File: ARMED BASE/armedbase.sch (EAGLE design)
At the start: 20 parts, among them IC1 REG1117, K1 CQ1-12V, X1 RJ45-6L2-B, X2 RJ45-6L2-B, X3 14867

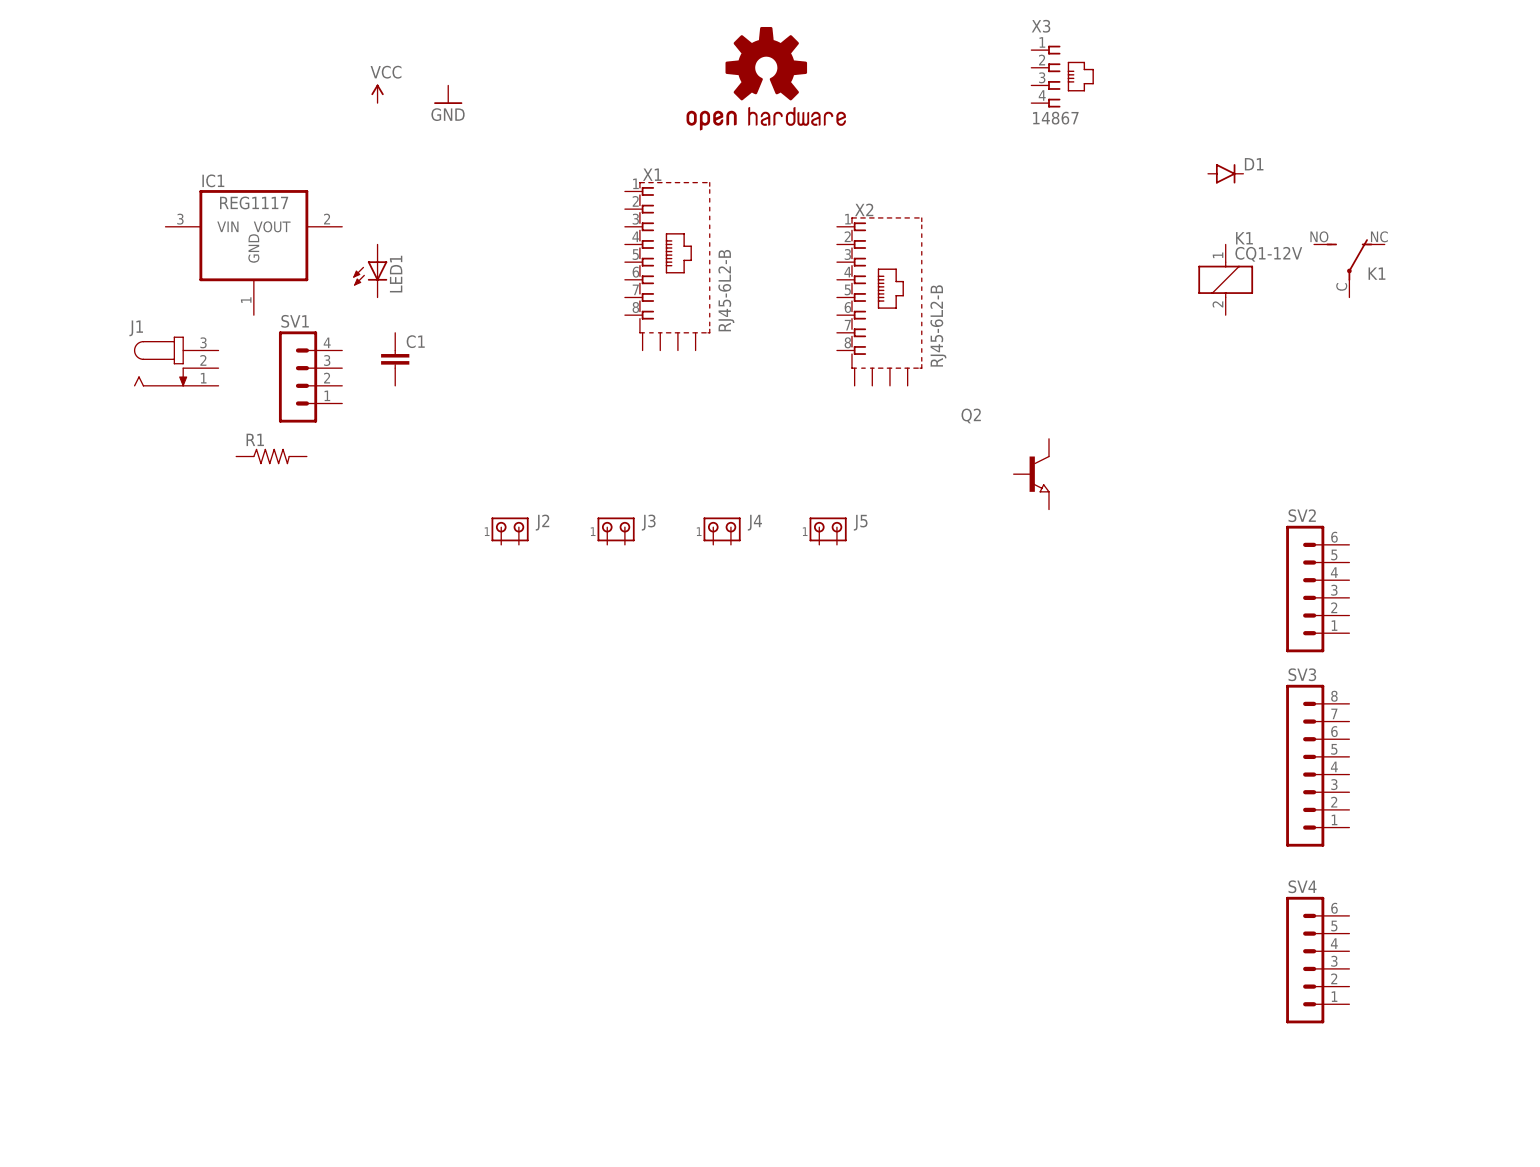
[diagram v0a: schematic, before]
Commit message: modbus
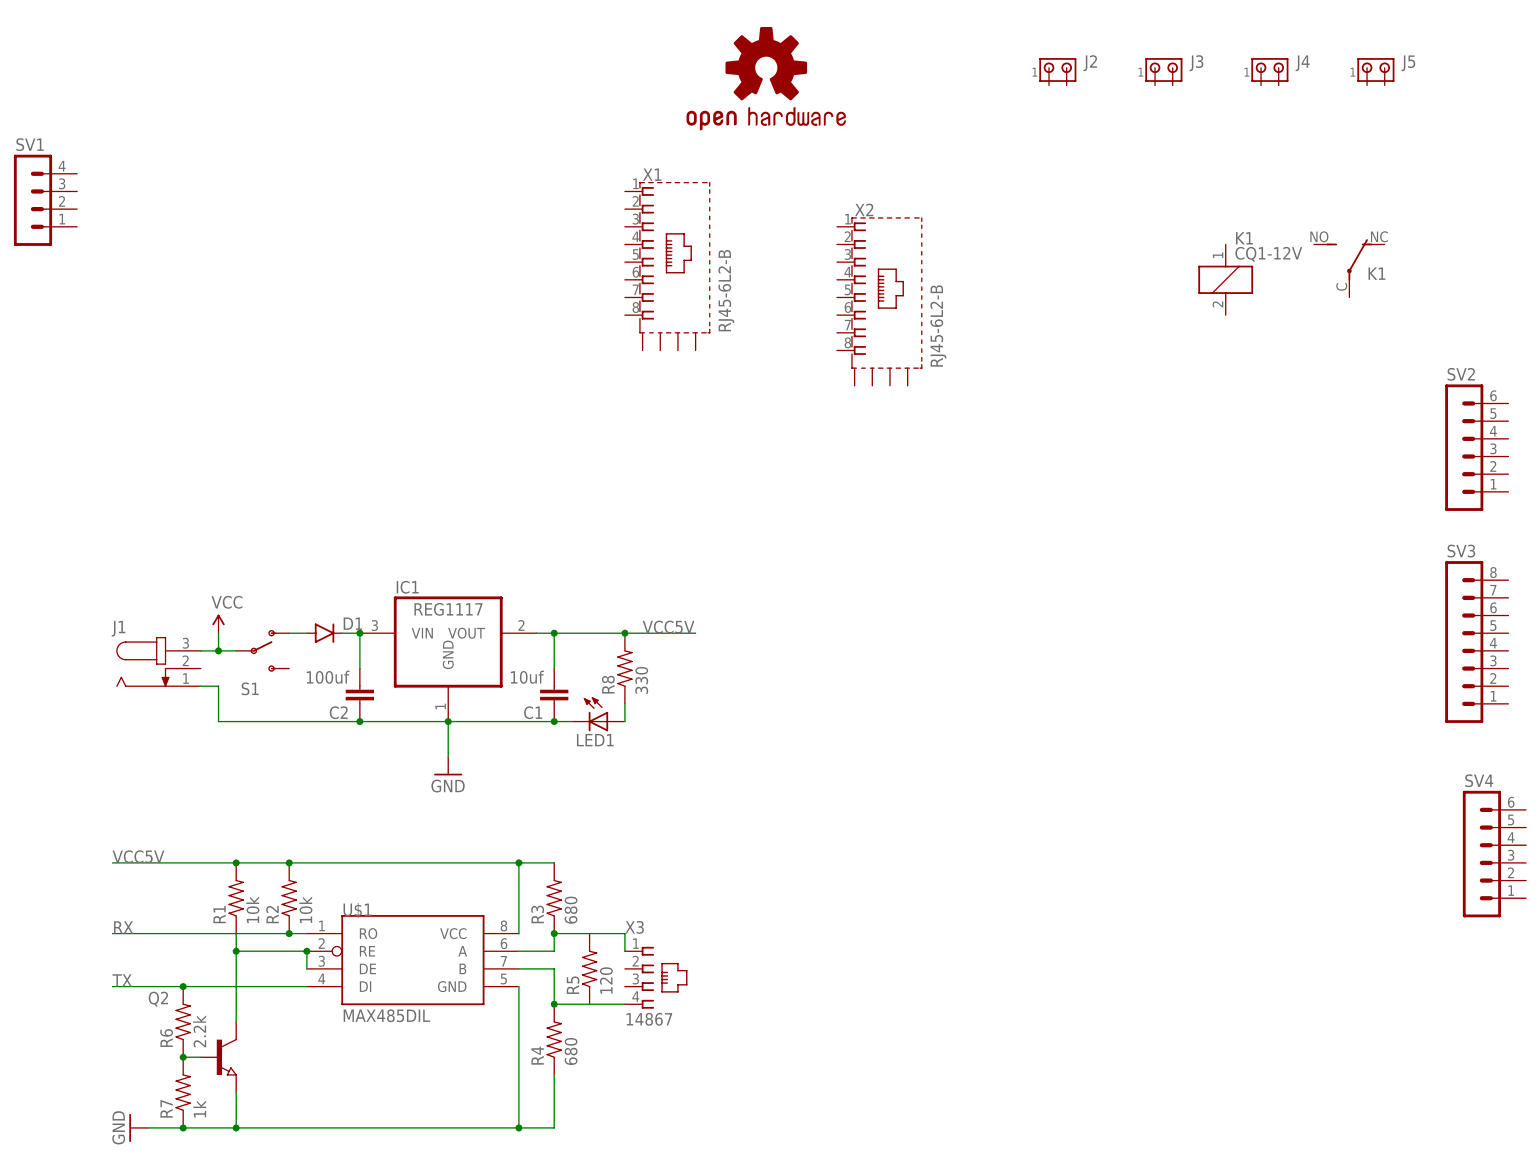
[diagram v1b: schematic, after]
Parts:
- added C2: 100uf, SparkFun-Capacitors:CAP0805
- added R2: 10k, SparkFun-Passives:RESISTOR0805-RES
- added R3, R4: 680, SparkFun-Passives:RESISTOR0805-RES
- added R5: 120, SparkFun-Passives:RESISTOR0805-RES
- added R6: 2.2k, SparkFun-Passives:RESISTOR0805-RES
- added R7: 1k, SparkFun-Passives:RESISTOR0805-RES
- added R8: 330, SparkFun-Passives:RESISTOR0805-RES
- added S1: (no value), SparkFun-Electromechanical:SWITCH-SPDTSMD2
- added U$1: MAX485DIL, SparkFun-DigitalIC:MAX485DIL
- C1: value (none) -> 10uf
- R1: value (none) -> 10k
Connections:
- new net GND: C1.1, C2.1, IC1.GND, J1.1, LED1.C, Q2.E, R4.1, R7.1, U$1.GND
- new net N$11: LED1.A, R8.1
- new net N$13: D1.A, S1.O
- new net N$14: C2.2, D1.C, IC1.VIN
- new net N$2: Q2.C, R1.1, U$1.DE, U$1.RE
- new net N$4: Q2.B, R6.1, R7.2
- new net N$7: R4.2, R5.1, U$1.B, X3.4
- new net N$8: R3.1, R5.2, U$1.A, X3.1
- new net RX: R2.1, U$1.RO
- new net TX: R6.2, U$1.DI
- new net VCC: J1.3, S1.P
- new net VCC5V: C1.2, IC1.VOUT, R1.2, R2.2, R3.2, R8.2, U$1.VCC
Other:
- moved on the sheet: C1, D1, IC1, J1, J2, J3, J4, J5, LED1, Q2, R1, SV1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
